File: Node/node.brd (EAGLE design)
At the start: 76.2 x 33.9 mm, 140 parts, among them J1 U.FL, J2 USBSMD, J3 U.FL, J5 CORTEX_DEBUGPTH, SW2 SPST_TACT-KMR2, U1 MCP73871, U2 DW1000-I, U3 RFM69HCW, U4 ATSAMD21G-A, U5 LSM303C, U6 LM3880, X2 332-02

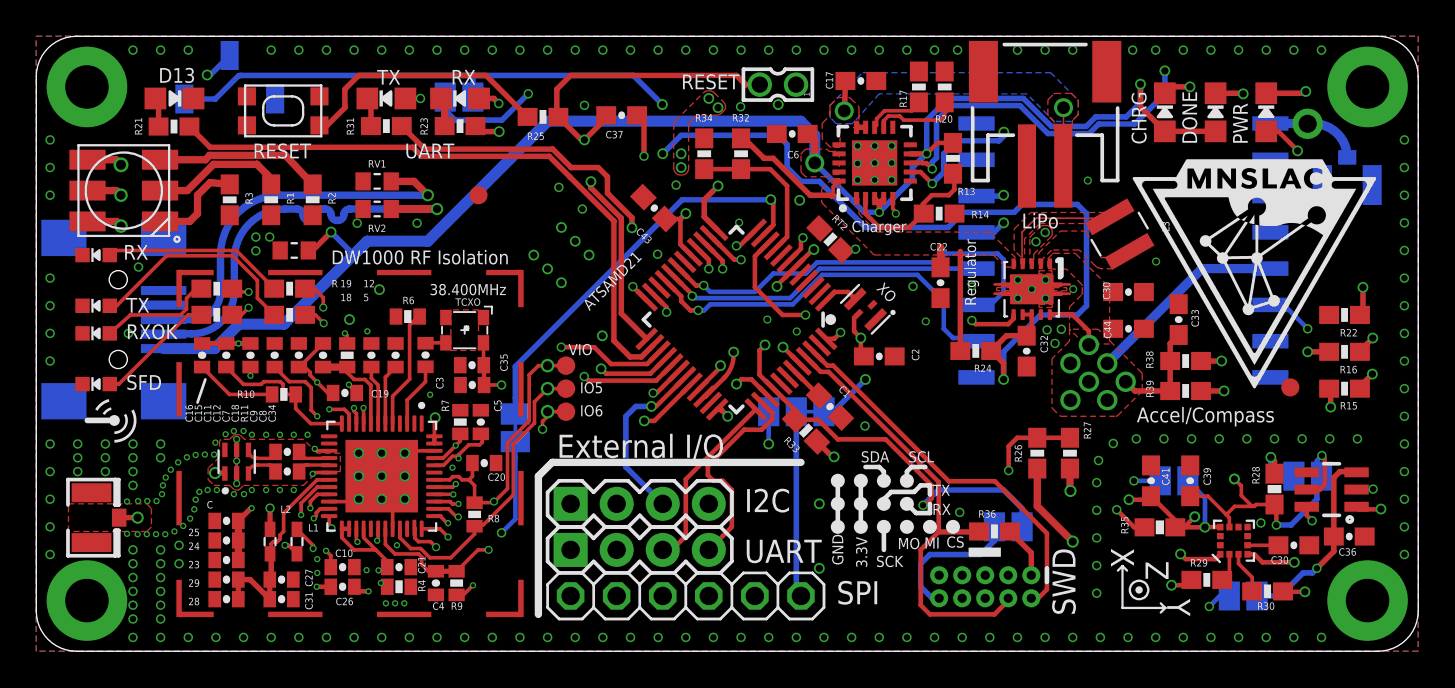
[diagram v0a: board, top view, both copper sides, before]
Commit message: Detailed changes, small stuff. Checking everything over. Switched to the new SAMD21 package.
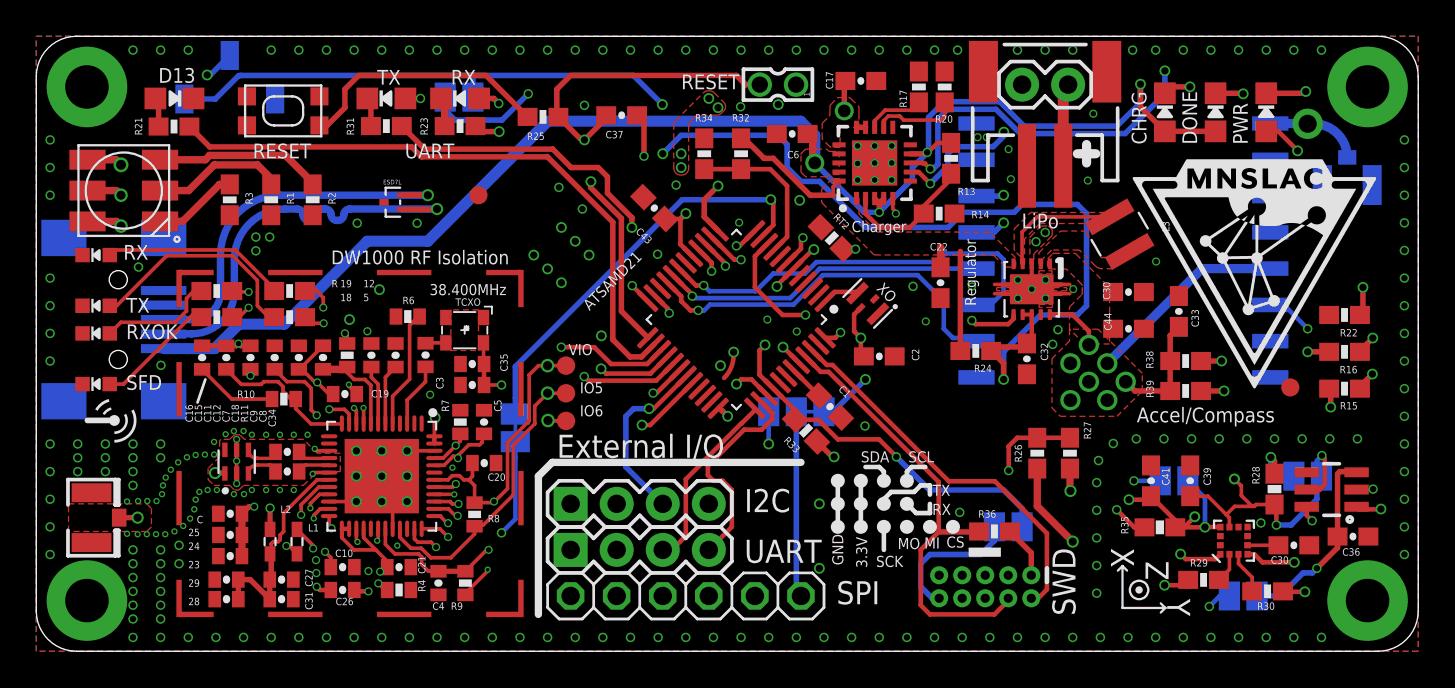
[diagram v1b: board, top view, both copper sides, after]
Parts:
- removed RV1, RV2, RV3: SUPPRESSOR-USB_0603_REFLOW, MainLib:WESURGE_0603_REFLOW
- added BOTTOM-LOGO: MNSLAC0.25, MainLib:MNSLAC-0.25
- added J4: (no value), SparkFun-Connectors:1X02
- added U$25: ESD7L, MainLib:SOT-723
- U$1: value MNSLAC0.25 -> FOUR_LAYER_WARNING; device MainLib:MNSLAC-0.25 -> SparkFun-Aesthetics:FOUR_LAYER_WARNING
- U2: device MainLib:QFN40P600X600X90-49N -> MainLib:QFN40P600X600X90-49T410
- U4: value ATSAMD21G-A -> SAMD21G18A-AUTTQFN48; device samd21:TQFP-48 -> MainLib:QFP50P900X900X120-48
- moved U$1 36.6 mm to (49.3, -4.06), flipped to the top
- moved TP2 0.51 mm to (29.2, 12.7)
- moved R9 0.48 mm to (23.7, 3.76)
- moved C44 0.45 mm to (63.0, 18.7)
- moved C25 0.44 mm to (10.7, 7.58)
- moved C32 0.43 mm to (54.6, 16.1)
- moved C24 0.37 mm to (10.7, 6.41)
- moved U$11 0.34 mm to (45.8, 19.2)
- moved C23 0.30 mm to (10.7, 5.25)
- moved R10 0.25 mm to (13.7, 13.9)
- moved TP1 0.25 mm to (29.2, 14.2)
- moved C36 0.20 mm to (72.6, 6.32)
- moved C5 0.18 mm to (24.7, 12.6)
- moved C26 0.18 mm to (16.9, 3.38)
- moved R4 0.18 mm to (20.0, 3.38)
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- renumbered U$14 to TOP-LOGO
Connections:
- net D+: now also U$25.P$2; no longer RV1.1
- net D-: now also U$25.P$1; no longer RV2.1
- net GND: now also J4.1, U$25.P$3; no longer RV1.2, RV2.2, RV3.2
- net VBUS: no longer RV3.1
- net VLIPO: now also J4.2
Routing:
- net VBUS: track 84.3 -> 79.7 mm, vias 5 -> 4
- net D-: track 43.3 -> 40.8 mm
- net D+: track 43.9 -> 41.5 mm
- net !RESET: track 60.2 -> 57.9 mm
- net GRN: track 39.0 -> 37.3 mm
- net VLIPO: track 5.38 -> 6.96 mm, vias 2 -> 1
- net GND: track 16.8 -> 18.1 mm, vias 269 -> 270
- net 3.3V: track 78.5 -> 79.4 mm
- net GPIO6: track 21.1 -> 21.9 mm, vias 4 -> 3
- net LSMVDDIO: track 39.6 -> 40.3 mm
- net N$4: track 5.33 -> 4.69 mm
- net N$8: track 8.17 -> 7.62 mm
- added copper zone on layer 15, net VLIPO
- removed copper zone on layer 16, net VLIPO
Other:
- board text added: "HS1"
- board text added: "HS2"
- board text added: "HS3"
- board text added: "HS4"
- board text added: "HS5"
- board text added: "MNSLAC Node PCB"
- board text removed: "RV1"
- board text removed: "RV2"
